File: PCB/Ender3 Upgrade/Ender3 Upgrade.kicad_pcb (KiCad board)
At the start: 2 copper layers, 95.5 x 118.9 mm, 1 part

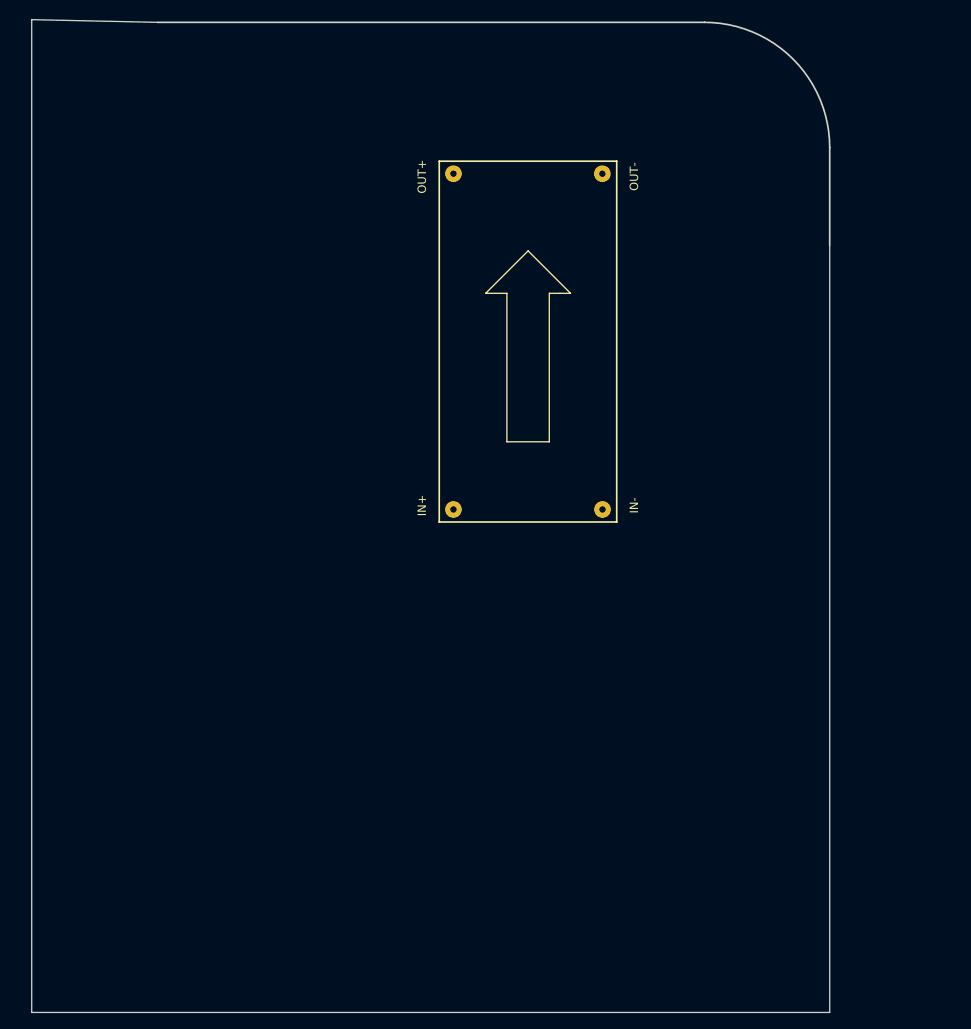
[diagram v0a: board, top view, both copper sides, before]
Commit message: LED Wire Clip
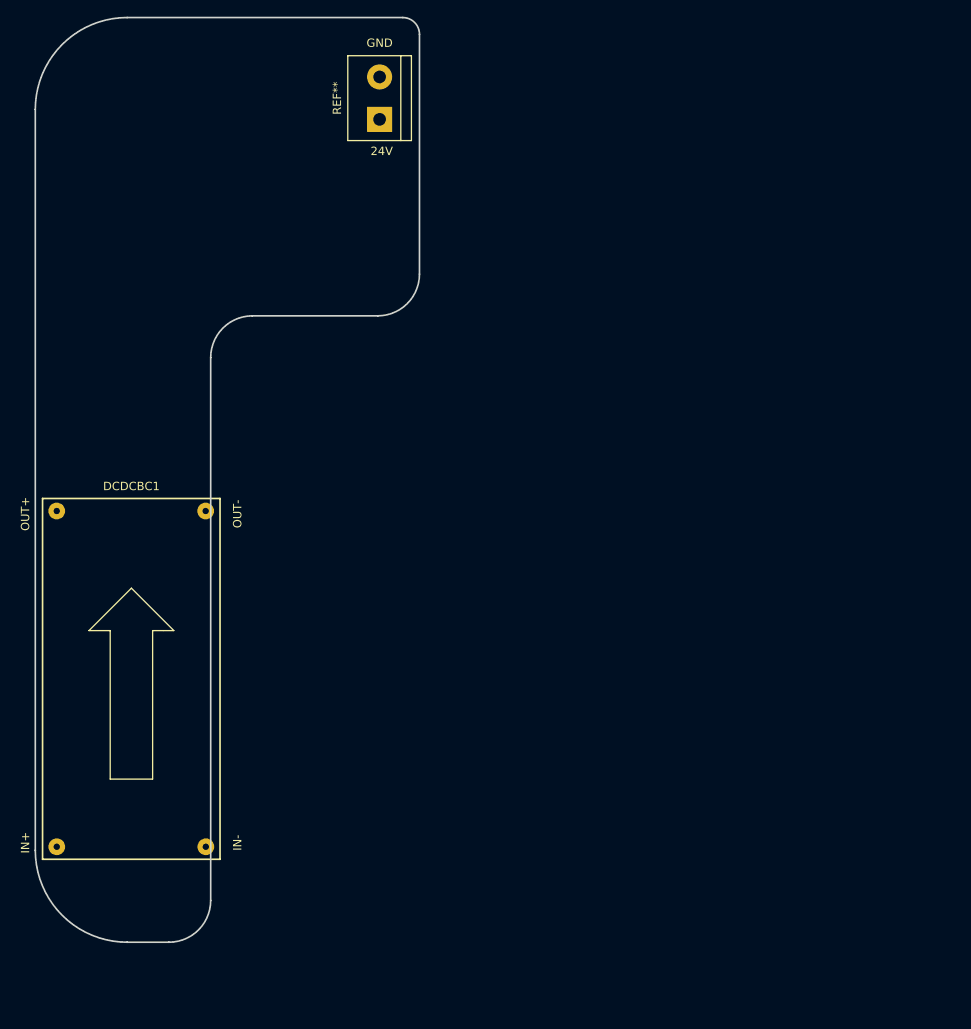
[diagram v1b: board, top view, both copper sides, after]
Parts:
- removed ?: BuckConverter, albe:BuckConverter
- added DCDCBC1: DCDCBuckConverter, albe:BuckConverter, F.Cu at (81.5, 120.1)
- added REF**: TerminalBlock_bornier-2_P5.08mm, TerminalBlock:TerminalBlock_bornier-2_P5.08mm, F.Cu at (111.3, 53.8)
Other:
- board size 95.5 x 118.9 mm -> 46 x 110.7 mm
- board text added: "24V"
- board text added: "GND"
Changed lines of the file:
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@@
   (general
     (thickness 1.6)
-    (drawings 18)
+    (drawings 14)
     (tracks 0)
     (zones 0)
-    (modules 1)
-    (nets 1)
+    (modules 2)
+    (nets 5)
   )
   (page A4)
@@
     (pad_drill 0.762)
     (pad_to_mask_clearance 0)
-    (aux_axis_origin 0 0)
-    (grid_origin 134.874 113.03)
-    (visible_elements FFFFFD7F)
+    (aux_axis_origin 18.796 151.638)
+    (grid_origin 43.942 185.166)
+    (visible_elements 7FFFFFFF)
     (pcbplotparams
       (layerselection 0x010fc_ffffffff)
@@
   )
   (net 0 "")
+  (net 1 "Net-(DCDCBC1-Pad4)")
+  (net 2 "Net-(DCDCBC1-Pad3)")
+  (net 3 +24V)
+  (net 4 GND)
   (net_class Default "This is the default net class."
     (clearance 0.2)
@@
     (uvia_dia 0.3)
     (uvia_drill 0.1)
+    (add_net +24V)
+    (add_net GND)
+    (add_net "Net-(DCDCBC1-Pad3)")
+    (add_net "Net-(DCDCBC1-Pad4)")
   )
   (module albe:BuckConverter (layer F.Cu)
-    (at 129.032 79.756)
-    (fp_text reference "" (at 0 -22.36) (layer F.SilkS)
-      (effects (font (size 1 1) (thickness 0.15)))
-    )
-    (fp_text value BuckConverter (at 0 -23.36) (layer F.Fab)
+    (at 81.534 120.142)
+    (fp_text reference DCDCBC1 (at 0 -22.36) (layer F.SilkS)
+      (effects (font (size 1 1) (thickness 0.15)))
+    )
+    (fp_text value DCDCBuckConverter (at 0 -23.36) (layer F.Fab)
       (effects (font (size 1 1) (thickness 0.15)))
     )
@@
     (fp_line (start 0 -10.16) (end 5.08 -5.08) (layer F.SilkS) (width 0.12))
     (fp_line (start 5.08 -5.08) (end 3.81 -5.08) (layer F.SilkS) (width 0.12))
-    (pad 4 thru_hole circle (at -8.939073 -19.398813) (size 2 2) (drill 0.762) (layers *.Cu *.Mask))
-    (pad 3 thru_hole circle (at 8.89 -19.398813) (size 2 2) (drill 0.762) (layers *.Cu *.Mask))
-    (pad 2 thru_hole circle (at -8.939073 20.801187) (size 2 2) (drill 0.762) (layers *.Cu *.Mask))
-    (pad 1 thru_hole circle (at 8.910927 20.801187) (size 2 2) (drill 0.762) (layers *.Cu *.Mask))
-  )
-  (gr_line (start 69.596 41.91) (end 84.665419 42.231605) (layer Edge.Cuts) (width 0.05))
-  (gr_line (start 69.596 160.782) (end 69.596 41.91) (layer Edge.Cuts) (width 0.05))
-  (gr_line (start 164.846 160.782) (end 69.596 160.782) (layer Edge.Cuts) (width 0.05))
-  (gr_line (start 165.146 160.782) (end 164.846 160.782) (layer Edge.Cuts) (width 0.05))
-  (gr_line (start 165.146 68.95) (end 165.146 160.782) (layer Edge.Cuts) (width 0.05))
-  (gr_circle (center 107.696 94.5) (end 106.296 94.5) (layer Dwgs.User) (width 0.2))
-  (gr_arc (start 150.146 145.95) (end 150.146 160.95) (angle -18.1761416) (layer Dwgs.User) (width 0.2))
-  (gr_line (start 84.665419 160.95) (end 150.146 160.95) (layer Dwgs.User) (width 0.2))
-  (gr_arc (start 84.665419 145.95) (end 69.665419 145.95) (angle -90) (layer Dwgs.User) (width 0.2))
-  (gr_arc (start 84.665419 57.231605) (end 84.665419 42.231605) (angle -90) (layer Dwgs.User) (width 0.2))
-  (gr_line (start 150.146 42.231605) (end 84.665419 42.231605) (layer Edge.Cuts) (width 0.2))
-  (gr_line (start 168.146 68.95) (end 165.146 68.95) (layer Dwgs.User) (width 0.2))
-  (gr_circle (center 156.596 94.5) (end 155.196 94.5) (layer Dwgs.User) (width 0.2))
-  (gr_circle (center 156.596 152.4) (end 155.196 152.4) (layer Dwgs.User) (width 0.2))
-  (gr_arc (start 150.146 57.231605) (end 165.146 57.231605) (angle -90) (layer Edge.Cuts) (width 0.2))
-  (gr_line (start 165.146 68.95) (end 165.146 57.231605) (layer Edge.Cuts) (width 0.2))
-  (gr_line (start 69.665419 57.231605) (end 69.665419 145.95) (layer Dwgs.User) (width 0.2))
-  (gr_circle (center 107.696 152.4) (end 106.296 152.4) (layer Dwgs.User) (width 0.2))
+    (pad 4 thru_hole circle (at -8.939073 -19.398813) (size 2 2) (drill 0.762) (layers *.Cu *.Mask)
+      (net 1 "Net-(DCDCBC1-Pad4)"))
+    (pad 3 thru_hole circle (at 8.89 -19.398813) (size 2 2) (drill 0.762) (layers *.Cu *.Mask)
+      (net 2 "Net-(DCDCBC1-Pad3)"))
+    (pad 2 thru_hole circle (at -8.939073 20.801187) (size 2 2) (drill 0.762) (layers *.Cu *.Mask)
+      (net 3 +24V))
+    (pad 1 thru_hole circle (at 8.910927 20.801187) (size 2 2) (drill 0.762) (layers *.Cu *.Mask)
+      (net 4 GND))
+  )
+  (module TerminalBlock:TerminalBlock_bornier-2_P5.08mm (layer F.Cu)
+    (at 111.252 53.848 90)
+    (descr "simple 2-pin terminal block, pitch 5.08mm, revamped version of bornier2")
+    (tags "terminal block bornier2")
+    (fp_text reference REF** (at 2.54 -5.08 90) (layer F.SilkS)
+      (effects (font (size 1 1) (thickness 0.15)))
+    )
+    (fp_text value TerminalBlock_bornier-2_P5.08mm (at 2.54 5.08 90) (layer F.Fab)
+      (effects (font (size 1 1) (thickness 0.15)))
+    )
+    (fp_text user %R (at 2.54 0 90) (layer F.Fab)
+      (effects (font (size 1 1) (thickness 0.15)))
+    )
+    (fp_line (start -2.41 2.55) (end 7.49 2.55) (layer F.Fab) (width 0.1))
+    (fp_line (start -2.46 -3.75) (end -2.46 3.75) (layer F.Fab) (width 0.1))
+    (fp_line (start -2.46 3.75) (end 7.54 3.75) (layer F.Fab) (width 0.1))
+    (fp_line (start 7.54 3.75) (end 7.54 -3.75) (layer F.Fab) (width 0.1))
+    (fp_line (start 7.54 -3.75) (end -2.46 -3.75) (layer F.Fab) (width 0.1))
+    (fp_line (start 7.62 2.54) (end -2.54 2.54) (layer F.SilkS) (width 0.12))
+    (fp_line (start 7.62 3.81) (end 7.62 -3.81) (layer F.SilkS) (width 0.12))
+    (fp_line (start 7.62 -3.81) (end -2.54 -3.81) (layer F.SilkS) (width 0.12))
+    (fp_line (start -2.54 -3.81) (end -2.54 3.81) (layer F.SilkS) (width 0.12))
+    (fp_line (start -2.54 3.81) (end 7.62 3.81) (layer F.SilkS) (width 0.12))
+    (fp_line (start -2.71 -4) (end 7.79 -4) (layer F.CrtYd) (width 0.05))
+    (fp_line (start -2.71 -4) (end -2.71 4) (layer F.CrtYd) (width 0.05))
+    (fp_line (start 7.79 4) (end 7.79 -4) (layer F.CrtYd) (width 0.05))
+    (fp_line (start 7.79 4) (end -2.71 4) (layer F.CrtYd) (width 0.05))
+    (pad 2 thru_hole circle (at 5.08 0 90) (size 3 3) (drill 1.52) (layers *.Cu *.Mask))
+    (pad 1 thru_hole rect (at 0 0 90) (size 3 3) (drill 1.52) (layers *.Cu *.Mask))
+    (model ${KISYS3DMOD}/TerminalBlock.3dshapes/TerminalBlock_bornier-2_P5.08mm.wrl
+      (offset (xyz 2.539999961853027 0 0))
+      (scale (xyz 1 1 1))
+      (rotate (xyz 0 0 0))
+    )
+  )
+  (gr_line (start 70.026 141.374395) (end 70.026 52.656) (layer Edge.Cuts) (width 0.2))
+  (gr_arc (start 81.026 52.656) (end 81.026 41.656) (angle -90) (layer Edge.Cuts) (width 0.2))
+  (gr_text 24V (at 111.506 57.658) (layer F.SilkS)
+    (effects (font (size 1 1) (thickness 0.15)))
+  )
+  (gr_text GND (at 111.252 44.704) (layer F.SilkS)
+    (effects (font (size 1 1) (thickness 0.15)))
+  )
+  (gr_arc (start 114.026 43.656) (end 116.026 43.656) (angle -90) (layer Edge.Cuts) (width 0.2))
+  (gr_arc (start 86.026 147.374395) (end 86.026 152.374395) (angle -90) (layer Edge.Cuts) (width 0.2))
+  (gr_line (start 111.026 77.374395) (end 96.026 77.374395) (layer Edge.Cuts) (width 0.2))
+  (gr_line (start 116.026 43.656) (end 116.026 72.374395) (layer Edge.Cuts) (width 0.2))
+  (gr_line (start 91.026 82.374395) (end 91.026 147.374395) (layer Edge.Cuts) (width 0.2))
+  (gr_arc (start 81.026 141.374395) (end 70.026 141.374395) (angle -90) (layer Edge.Cuts) (width 0.2))
+  (gr_line (start 86.026 152.374395) (end 81.026 152.374395) (layer Edge.Cuts) (width 0.2))
+  (gr_arc (start 96.026 82.374395) (end 96.026 77.374395) (angle -90) (layer Edge.Cuts) (width 0.2))
+  (gr_arc (start 111.026 72.374395) (end 111.026 77.374395) (angle -90) (layer Edge.Cuts) (width 0.2))
+  (gr_line (start 81.026 41.656) (end 114.026 41.656) (layer Edge.Cuts) (width 0.2))
 )

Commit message: PCB Designed
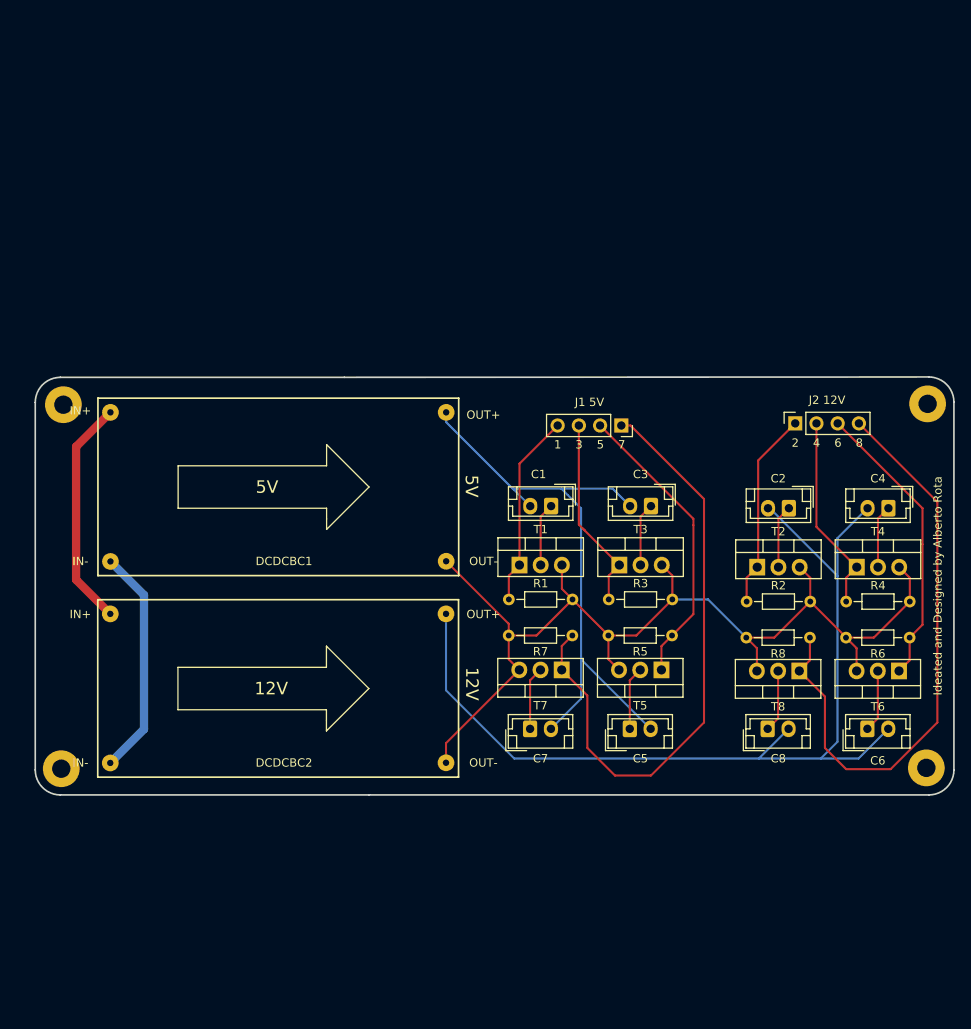
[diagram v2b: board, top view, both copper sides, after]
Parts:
- removed the REF** at (111.3, 53.8)
- added C1: Conn_01x02, Connector_JST:JST_EH_B2B-EH-A_1x02_P2.50mm_Vertical, F.Cu at (131.8, 100.2)
- added C2: Conn_01x02, Connector_JST:JST_EH_B2B-EH-A_1x02_P2.50mm_Vertical, F.Cu at (160.3, 100.4)
- added C3: Conn_01x02, Connector_JST:JST_EH_B2B-EH-A_1x02_P2.50mm_Vertical, F.Cu at (143.7, 100.2)
- added C4: Conn_01x02, Connector_JST:JST_EH_B2B-EH-A_1x02_P2.50mm_Vertical, F.Cu at (172.2, 100.4)
- added C5: Conn_01x02, Connector_JST:JST_EH_B2B-EH-A_1x02_P2.50mm_Vertical, F.Cu at (141.2, 126.8)
- added C6: Conn_01x02, Connector_JST:JST_EH_B2B-EH-A_1x02_P2.50mm_Vertical, F.Cu at (169.7, 126.8)
- added C7: Conn_01x02, Connector_JST:JST_EH_B2B-EH-A_1x02_P2.50mm_Vertical, F.Cu at (129.3, 126.8)
- added C8: Conn_01x02, Connector_JST:JST_EH_B2B-EH-A_1x02_P2.50mm_Vertical, F.Cu at (157.7, 126.8)
- added DCDCBC2: DCDC 24-12, albe:BuckConverter, F.Cu at (99.8, 122.0)
- added J1 5V: Conn_01x04_Male, Connector_PinSocket_2.54mm:PinSocket_1x04_P2.54mm_Vertical, F.Cu at (140.2, 90.5)
- added J2 12V: Conn_01x04_Male, Connector_PinSocket_2.54mm:PinSocket_1x04_P2.54mm_Vertical, F.Cu at (161.0, 90.2)
- added R1: R1, Resistor_THT:R_Axial_DIN0204_L3.6mm_D1.6mm_P7.62mm_Horizontal, F.Cu at (126.7, 111.3)
- added R2: R1, Resistor_THT:R_Axial_DIN0204_L3.6mm_D1.6mm_P7.62mm_Horizontal, F.Cu at (155.2, 111.6)
- added R3: R1, Resistor_THT:R_Axial_DIN0204_L3.6mm_D1.6mm_P7.62mm_Horizontal, F.Cu at (138.7, 111.3)
- added R4: R1, Resistor_THT:R_Axial_DIN0204_L3.6mm_D1.6mm_P7.62mm_Horizontal, F.Cu at (167.1, 111.6)
- added R5: R1, Resistor_THT:R_Axial_DIN0204_L3.6mm_D1.6mm_P7.62mm_Horizontal, F.Cu at (146.3, 115.6)
- added R6: R1, Resistor_THT:R_Axial_DIN0204_L3.6mm_D1.6mm_P7.62mm_Horizontal, F.Cu at (174.7, 115.9)
- added R7: R1, Resistor_THT:R_Axial_DIN0204_L3.6mm_D1.6mm_P7.62mm_Horizontal, F.Cu at (134.3, 115.6)
- added R8: R1, Resistor_THT:R_Axial_DIN0204_L3.6mm_D1.6mm_P7.62mm_Horizontal, F.Cu at (162.8, 115.9)
- added REF**: MountingHole_2.2mm_M2_Pad, MountingHole:MountingHole_2.2mm_M2_Pad, F.Cu at (176.9, 87.9)
- added REF**: MountingHole_2.2mm_M2_Pad, MountingHole:MountingHole_2.2mm_M2_Pad, F.Cu at (176.7, 131.5)
- added REF**: MountingHole_2.2mm_M2_Pad, MountingHole:MountingHole_2.2mm_M2_Pad, F.Cu at (73.1, 131.6)
- added REF**: MountingHole_2.2mm_M2_Pad, MountingHole:MountingHole_2.2mm_M2_Pad, F.Cu at (73.4, 88.0)
- added T1: IRLZ34N, Package_TO_SOT_THT:TO-220-3_Vertical, F.Cu at (128.0, 107.2)
- added T2: IRLZ34N, Package_TO_SOT_THT:TO-220-3_Vertical, F.Cu at (156.5, 107.5)
- added T3: IRLZ34N, Package_TO_SOT_THT:TO-220-3_Vertical, F.Cu at (140.0, 107.2)
- added T4: IRLZ34N, Package_TO_SOT_THT:TO-220-3_Vertical, F.Cu at (168.4, 107.5)
- added T5: IRLZ34N, Package_TO_SOT_THT:TO-220-3_Vertical, F.Cu at (145.0, 119.8)
- added T6: IRLZ34N, Package_TO_SOT_THT:TO-220-3_Vertical, F.Cu at (173.4, 119.9)
- added T7: IRLZ34N, Package_TO_SOT_THT:TO-220-3_Vertical, F.Cu at (133.1, 119.8)
- added T8: IRLZ34N, Package_TO_SOT_THT:TO-220-3_Vertical, F.Cu at (161.5, 119.9)
- DCDCBC1: value DCDCBuckConverter -> DCDC 24-5
- moved DCDCBC1 28.8 mm to (99.8, 97.9), turned to 270 degrees
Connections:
- DCDCBC1 pad 1: GND -> GNDPWR
- DCDCBC1 pad 3: Net-(DCDCBC1-Pad3) -> GND
- DCDCBC1 pad 4: Net-(DCDCBC1-Pad4) -> 5V
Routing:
- net GND: track 0.00 -> 124.7 mm
- net 12V: track 0.00 -> 116.0 mm
- net 5V: track 0.00 -> 73.6 mm
- net Net-(J1-Pad1): track 0.00 -> 73.5 mm
- net Net-(J2-Pad4): track 0.00 -> 71.5 mm
- net Net-(J1-Pad2): track 0.00 -> 35.5 mm
- net Net-(J2-Pad3): track 0.00 -> 35.0 mm
- net +24V: track 0.00 -> 27.5 mm
- net GNDPWR: track 0.00 -> 27.5 mm
- net Net-(J2-Pad2): track 0.00 -> 23.9 mm
- net Net-(J2-Pad1): track 0.00 -> 23.7 mm
- net Net-(J1-Pad3): track 0.00 -> 23.6 mm
- net Net-(J1-Pad4): track 0.00 -> 23.4 mm
- net Net-(C3-Pad1): track 0.00 -> 7.58 mm
- net Net-(C1-Pad1): track 0.00 -> 7.58 mm
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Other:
- board size 46 x 110.7 mm -> 110 x 50 mm
- board text added: "1"
- board text added: "12V"
- board text added: "2"
- board text added: "3"
- board text added: "4"
- board text added: "5"
- board text added: "5V"
- board text added: "6"
- board text added: "7"
- board text added: "8"
- board text added: "Ideated and Designed by Alberto Rota"
- board text removed: "24V"
- board text removed: "GND"
